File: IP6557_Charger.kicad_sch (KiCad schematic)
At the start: 44 parts, among them J1 Conn_01x04, J2 XKB_U262-16XN, Q1 CSD17581Q3A, Q2 CSD17581Q3A, Q3 CSD17581Q3A, Q4 CSD17581Q3A, U1 IP6557_C, U2 ESD224DQA

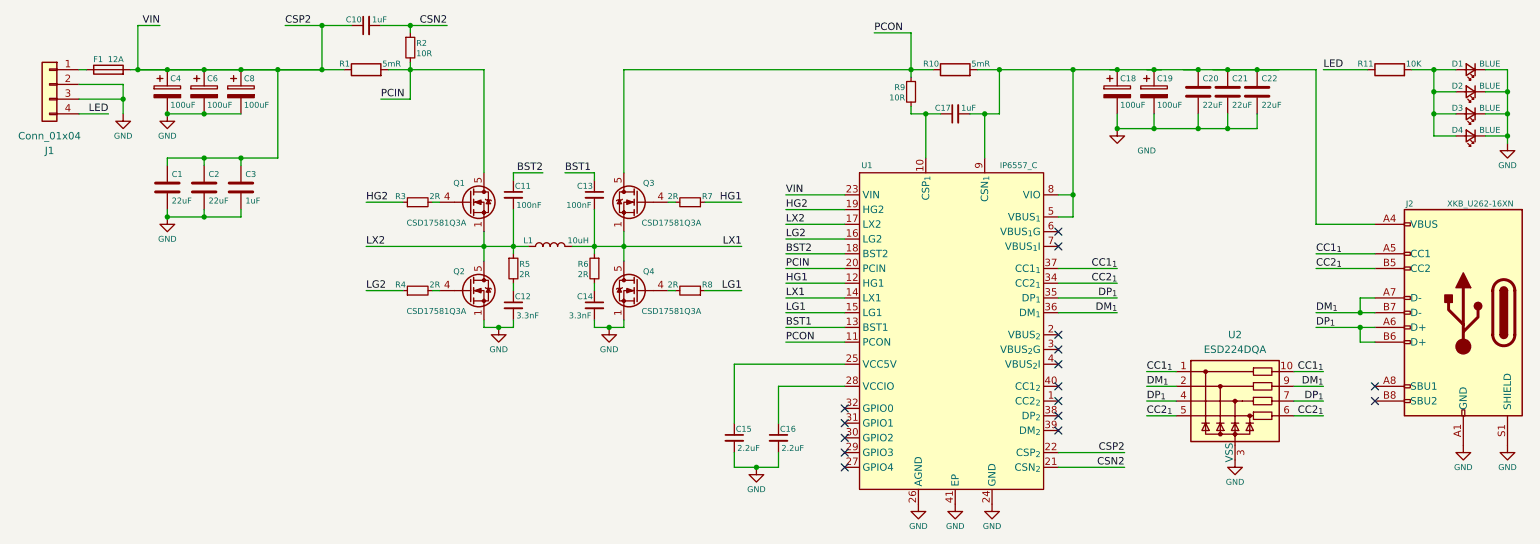
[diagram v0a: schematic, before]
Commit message: Upd
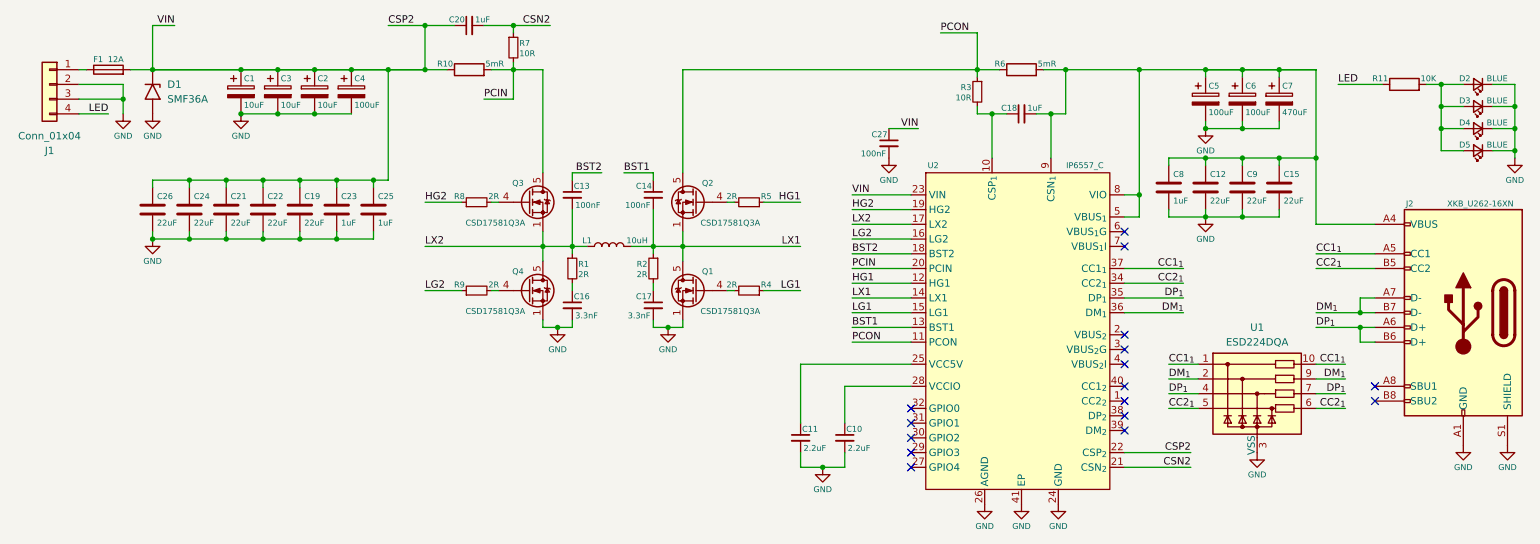
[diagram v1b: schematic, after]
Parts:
- added C19, C21, C22: 22uF, Capacitor_SMD:C_0805_2012Metric, symbol Device:C
- added C25: 1uF, Capacitor_SMD:C_0603_1608Metric, symbol Device:C
- added C27: 100nF, Capacitor_SMD:C_0402_1005Metric, symbol Device:C_Small
- added C4: 100uF, IP6557_Charger:CP_Radial_D5.0mm_P2.00mm, symbol Device:C_Polarized
- added C7: 470uF, IP6557_Charger:CP_Radial_D8.0mm_P3.50mm, symbol Device:C_Polarized
- added C8: 1uF, Capacitor_SMD:C_0805_2012Metric, symbol Device:C
- added D1: SMF36A, Diode_SMD:D_SMF, symbol Diode:SMF36A
- C1: renamed from C4; value 100uF -> 10uF
- C2: renamed from C8; value 100uF -> 10uF
- C3: renamed from C6; value 100uF -> 10uF
- F1: footprint Fuse:Fuse_0805_2012Metric -> Fuse:Fuse_1206_3216Metric
- renumbered C16 to C10, C15 to C11, C20 to C12, C11 to C13, C13 to C14, C22 to C15, C12 to C16, C14 to C17, C17 to C18, C10 to C20, C3 to C23, C2 to C24, C1 to C26, C18 to C5, C19 to C6, C21 to C9, D1 to D2, D2 to D3, D3 to D4, D4 to D5, Q4 to Q1, Q3 to Q2, Q1 to Q3, Q2 to Q4, R5 to R1, R1 to R10, R6 to R2, R9 to R3, R8 to R4, R7 to R5, R10 to R6, R2 to R7, R3 to R8, R4 to R9, U2 to U1, U1 to U2
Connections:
- net CSP2: now also C19.1, C21.1, C22.1, C25.1, C27.1, C4.1, D1.1 (A1)
- net GND: now also C19.2, C21.2, C22.2, C25.2, C27.2, C4.2, C7.2, C8.2, D1.2 (A2)
- net at C12.1, C15.1, C18.2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: now also C7.1, C8.1
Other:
- moved on the sheet: C1, C10, C11, C12, C13, C14, C15, C16, C17, C18, C2, C20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
